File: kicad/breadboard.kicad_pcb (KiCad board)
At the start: 2 copper layers, 83.8 x 58.4 mm, 9 parts

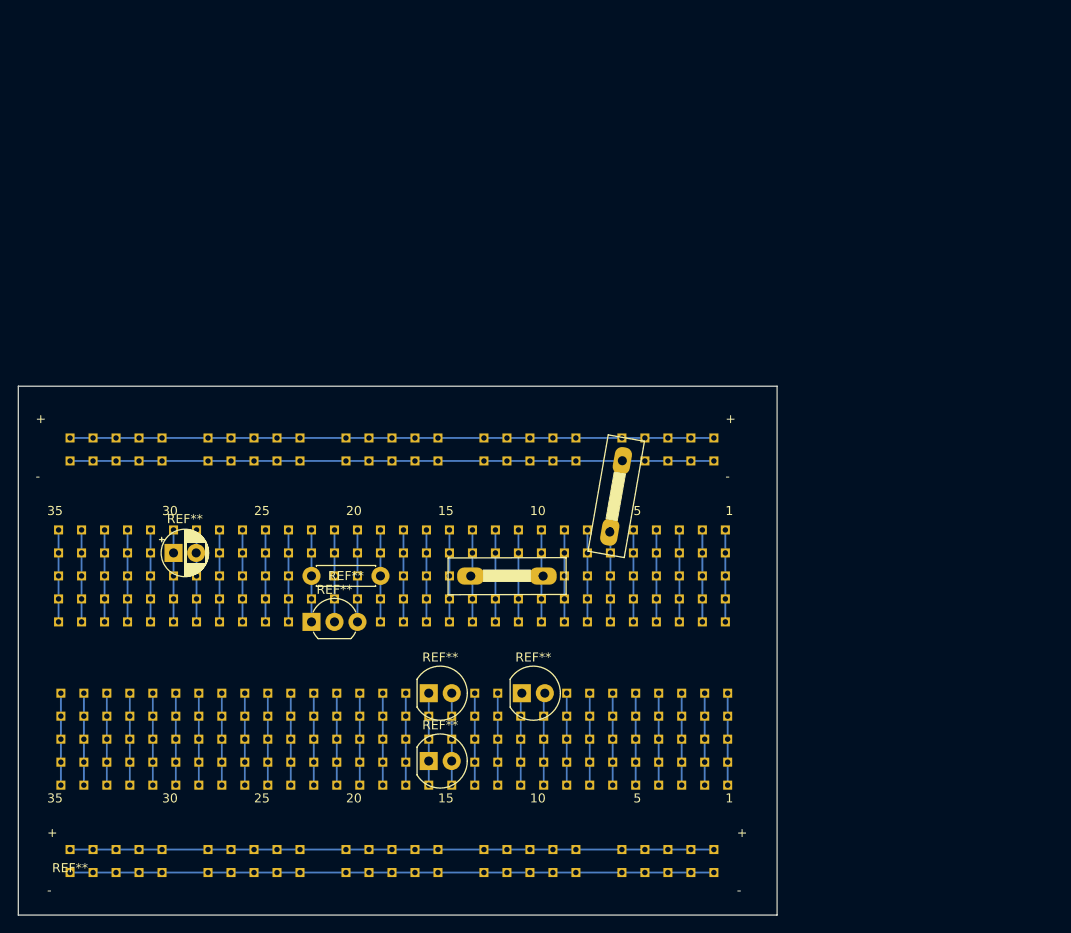
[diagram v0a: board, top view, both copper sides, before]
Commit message: some kicad stuff 🐟 🐟 🐟 🐟 🐟 🐟 🐟 🐟 🐟 🐟 🐟 🐟 🐟 🐟 🐟 🐟 :fish:
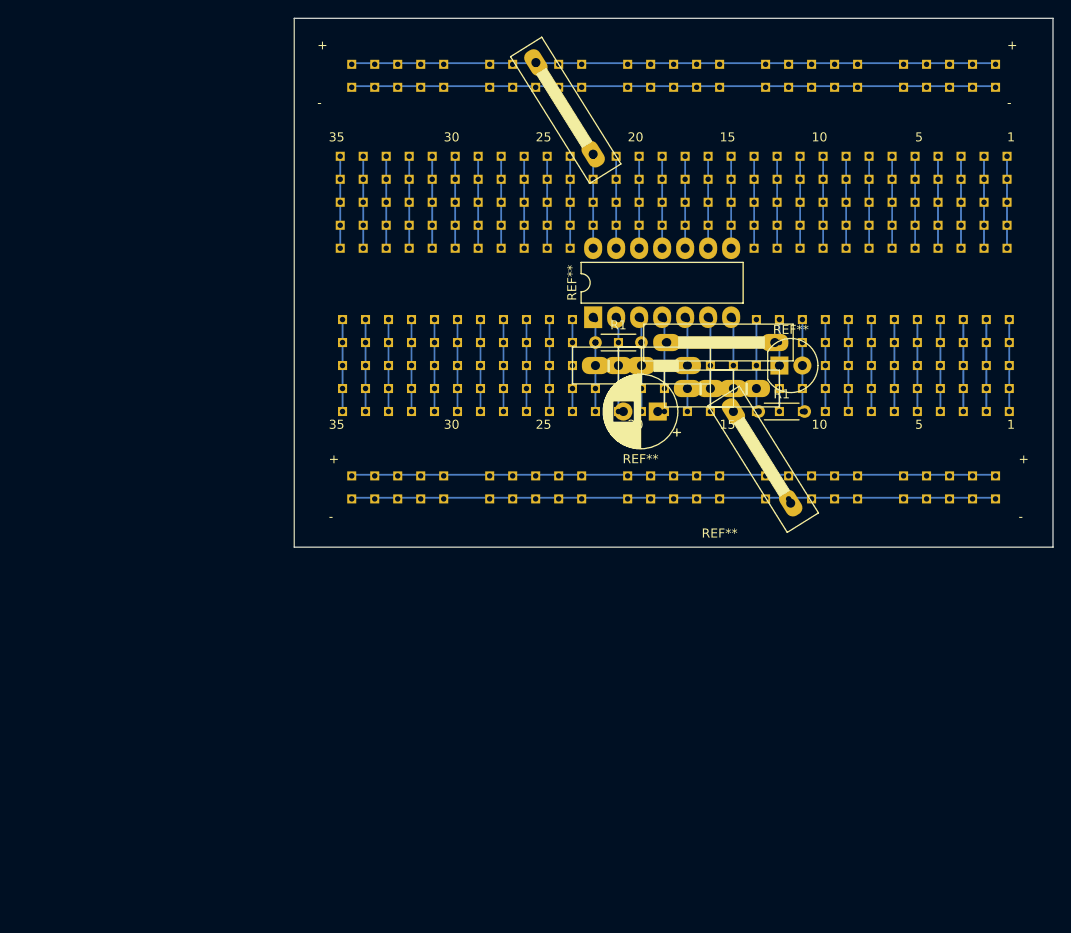
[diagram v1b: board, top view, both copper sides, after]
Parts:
- removed the REF** at (167.2, 120.0)
- removed the REF** at (149.2, 120.0)
- removed the REF** at (126.4, 117.5)
- removed the REF** at (141.6, 125.1)
- removed the REF** at (164.8, 133.0)
- removed the REF** at (154.6, 133.0)
- removed the REF** at (154.6, 140.5)
- removed the REF** at (175.9, 107.3)
- added R1: 100k, Resistor_THT:R_Axial_DIN0204_L3.6mm_D1.6mm_P5.08mm_Horizontal, F.Cu at (173.0, 94.2)
- added R1: 100k, Resistor_THT:R_Axial_DIN0204_L3.6mm_D1.6mm_P5.08mm_Horizontal, F.Cu at (191.0, 101.9)
- added REF**: Jumper-Wire_12mm_Blue, Breadboarding:Jumper-Wire_12mm_Blue, F.Cu at (194.5, 112.0)
- added REF**: Jumper-Wire_5mm_Blue, Breadboarding:Jumper-Wire_5mm_Blue, F.Cu at (178.1, 96.8)
- added REF**: Jumper-Wire_12mm_Blue, Breadboarding:Jumper-Wire_12mm_Blue, F.Cu at (180.8, 94.2)
- added REF**: DIP-14_W7.62mm_LongPads, EZ_TEJ_Library:DIP-14_W7.62mm_LongPads, F.Cu at (172.7, 91.4)
- added REF**: Jumper-Wire_2.5mm_Blue, Breadboarding:Jumper-Wire_2.5mm_Blue, F.Cu at (183.1, 99.3)
- added REF**: LED_D5.0mm, EZ_TEJ_Library:LED_D5.0mm, F.Cu at (193.3, 96.8)
- added REF**: CP_Radial_D8.0mm_P3.80mm, EZ_TEJ_Library:CP_Radial_D8.0mm_P3.80mm, F.Cu at (179.9, 101.9)
- added REF**: Jumper-Wire_2.5mm_Blue, Breadboarding:Jumper-Wire_2.5mm_Blue, F.Cu at (173.0, 96.8)
- added REF**: Jumper-Wire_12mm_Blue, Breadboarding:Jumper-Wire_12mm_Blue, F.Cu at (172.7, 73.4)
- added REF**: Jumper-Wire_2.5mm_Blue, Breadboarding:Jumper-Wire_2.5mm_Blue, F.Cu at (188.2, 99.3)
- moved REF** 51.7 mm to (146.1, 111.5)
